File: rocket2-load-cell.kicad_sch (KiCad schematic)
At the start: 36 parts, among them J1 SWD, J2 Screw_Terminal_01x02, U2 STM32F103C8Tx, U3 AMS1117-3.3, Y1 16MHz

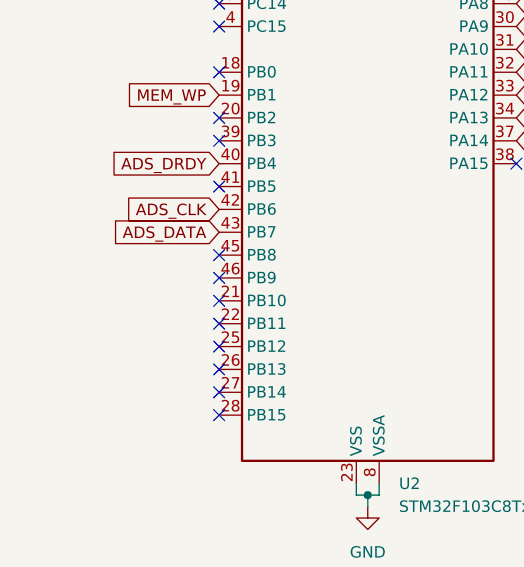
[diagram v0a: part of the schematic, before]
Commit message: added code and stab
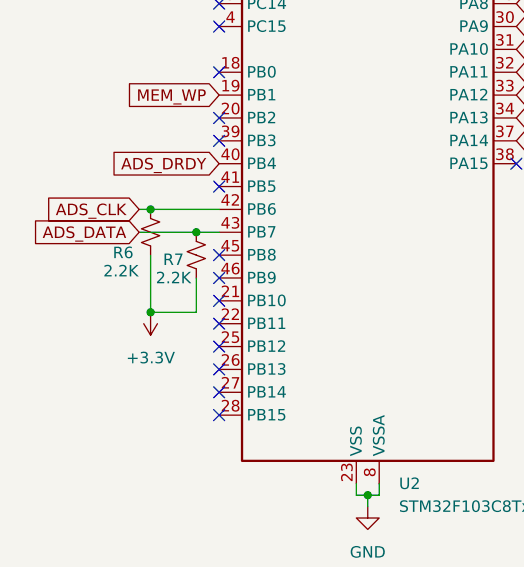
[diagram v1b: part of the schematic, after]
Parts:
- added R6, R7: 2.2K, Resistor_SMD:R_0603_1608Metric, symbol Device:R_Small_US
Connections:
- net +3.3V: now also R6.1, R7.1
- net ADS_CLK: now also R6.2
- net ADS_DATA: now also R7.2
